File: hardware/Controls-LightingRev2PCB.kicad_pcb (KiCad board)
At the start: 2 copper layers, 54.5 x 53.5 mm, 52 parts, among them IC1 LM74502HDDFR, IC3 ACS724LLCTR-05AU-T, IC4 ACS724LLCTR-05AU-T, IC5 TLV70433DBVT, IC6 ACS724LLCTR-05AU-T, J1 53307-2471, J3 Conn_02x05_Top_Bottom, J4 Conn_01x02, J5 Conn_01x02, J6 Conn_01x03, Q1 NVMFWS1D7N04XMT1G, Q3 IRLML0030, Q4 NVMFWS1D7N04XMT1G, Q5 IRLML0030, U5 SN74LV1T34DBV

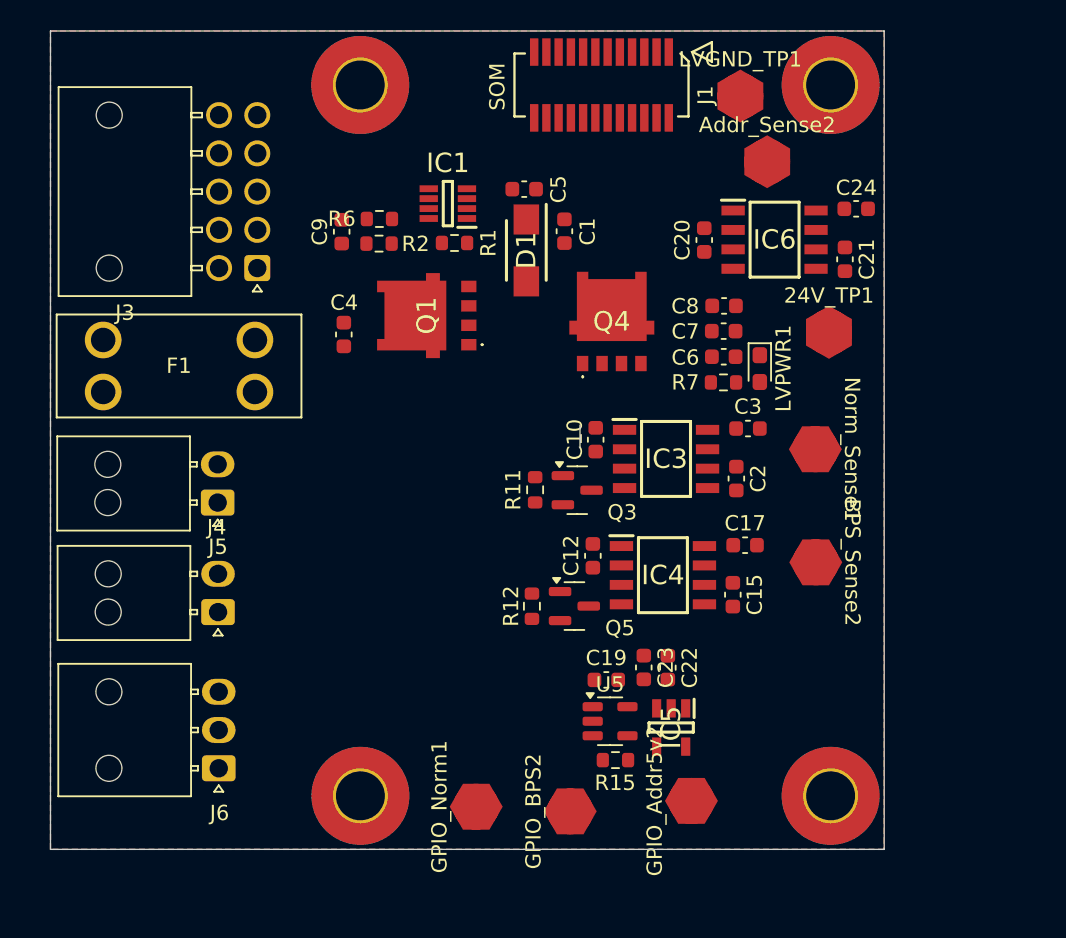
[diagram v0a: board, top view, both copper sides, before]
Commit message: Some routing
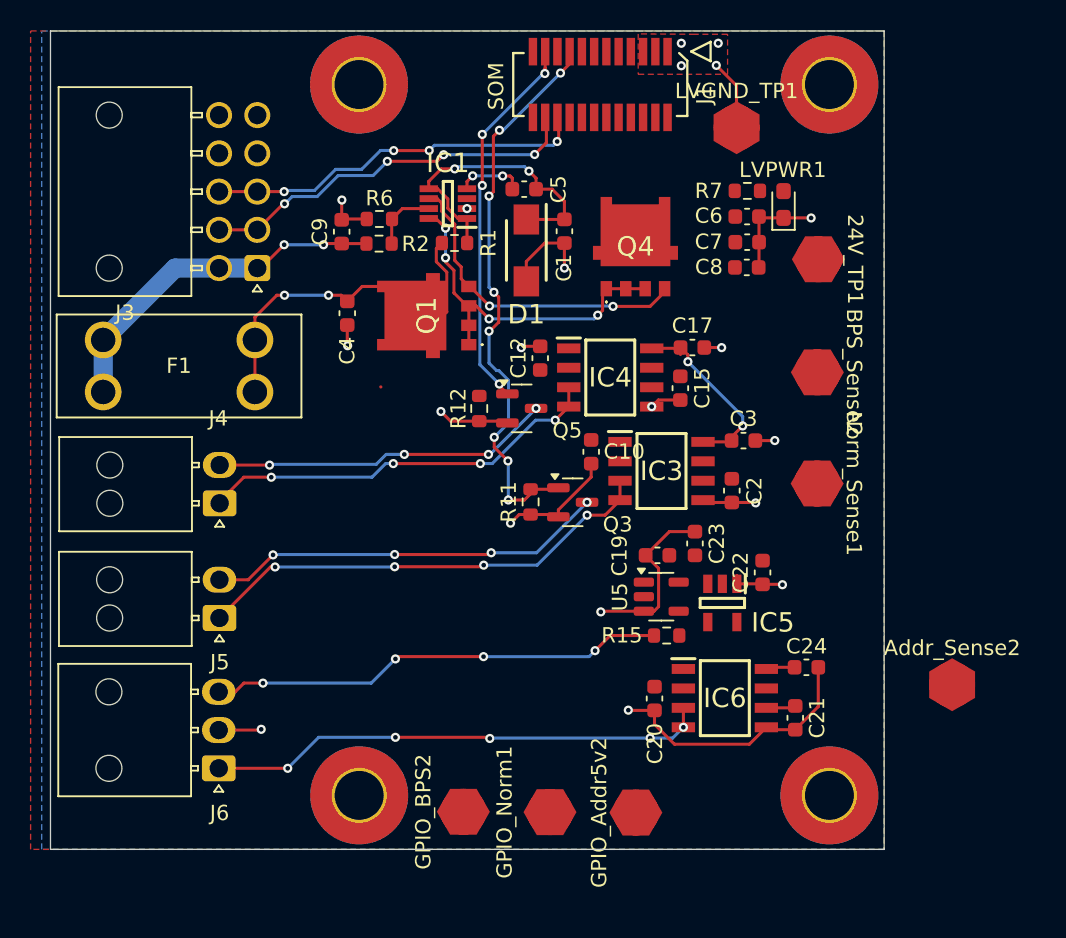
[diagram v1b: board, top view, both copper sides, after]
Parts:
- moved Addr_Sense2 36.3 mm to (232.9, 127.7)
- moved C20 30.1 mm to (213.5, 128.6)
- moved C24 30.1 mm to (223.4, 126.6)
- moved C21 30.1 mm to (222.7, 129.9)
- moved IC6 30.1 mm to (218.1, 128.6)
- moved C15 13.9 mm to (215.2, 108.3)
- moved R12 13.4 mm to (202.0, 109.7)
- moved C12 13.4 mm to (206.0, 106.4)
- moved C17 13.4 mm to (216.0, 105.7)
- moved IC4 13.4 mm to (210.6, 107.7)
- moved Q5 13.4 mm to (204.8, 109.7)
- moved R7 12.6 mm to (219.6, 95.5), turned to 0 degrees
- moved BPS_Sense2 12.4 mm to (224.1, 107.3)
- moved LVPWR1 10.8 mm to (221.9, 96.3), turned to 90 degrees
- moved C6 9.29 mm to (219.5, 97.1), turned to 0 degrees
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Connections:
- 24V_TP1 pad 1: Addressable_PWR -> +24V
- C1 pad 1: Addressable_GND -> GND
- C10 pad 1: Addressable_GND -> GND
- C10 pad 2: Addressable_PWR -> +24V
- C12 pad 1: Addressable_GND -> GND
- C12 pad 2: Addressable_PWR -> +24V
- C15 pad 2: Addressable_GND -> GND
- C17 pad 2: Addressable_GND -> GND
- C19 pad 1: Addressable_GND -> GND
- C2 pad 2: Addressable_GND -> GND
- C20 pad 1: Addressable_GND -> GND
- C20 pad 2: Addressable_PWR -> +24V
- C21 pad 2: Addressable_GND -> GND
- C22 pad 1: Addressable_GND -> GND
- C22 pad 2: Addressable_PWR -> +24V
- C23 pad 1: Addressable_GND -> GND
- C24 pad 2: Addressable_GND -> GND
- C3 pad 2: Addressable_GND -> GND
- C4 pad 2: Addressable_GND -> GND
- C6 pad 1: Addressable_PWR -> +24V
- C6 pad 2: Addressable_GND -> GND
- C7 pad 1: Addressable_PWR -> +24V
- C7 pad 2: Addressable_GND -> GND
- C8 pad 1: Addressable_PWR -> +24V
- C8 pad 2: Addressable_GND -> GND
- C9 pad 2: Addressable_GND -> GND
- D1 pad 2: Addressable_GND -> GND
- IC1 pad 2: Addressable_GND -> GND
- IC3 pad 1: Addressable_PWR -> +24V
- IC3 pad 2: Addressable_PWR -> +24V
- IC3 pad 3: Normal_GND -> Net-(IC3-IP-_1)
- IC3 pad 4: Normal_GND -> Net-(IC3-IP-_1)
- IC3 pad 5: Addressable_GND -> GND
- IC4 pad 1: Addressable_PWR -> +24V
- IC4 pad 2: Addressable_PWR -> +24V
- IC4 pad 3: Strobe_GND -> Net-(IC4-IP-_1)
- IC4 pad 4: Strobe_GND -> Net-(IC4-IP-_1)
- IC4 pad 5: Addressable_GND -> GND
- IC5 pad 1: Addressable_GND -> GND
- IC5 pad 2: Addressable_PWR -> +24V
- IC6 pad 1: Addressable_PWR -> +24V
- IC6 pad 2: Addressable_PWR -> +24V
- IC6 pad 3: Addressable_GND -> Net-(IC6-IP-_1)
- IC6 pad 4: Addressable_GND -> Net-(IC6-IP-_1)
- IC6 pad 5: Addressable_GND -> GND
- J1 pad 1: Addressable_GND -> GND
- J1 pad 24: Addressable_PWR -> +24V
- J1 pad 3: Addressable_GND -> GND
- J1 pad 5: Addressable_GND -> GND
- J3 pad 10: Addressable_GND -> GND
- J3 pad 4: Addressable_GND -> GND
- J3 pad 5: Addressable_GND -> GND
- J3 pad 9: Addressable_GND -> GND
- J4 pad 1: Addressable_PWR -> Net-(IC4-IP-_1)
- J4 pad 2: Strobe_GND -> Net-(J4-Pin_2)
- J5 pad 1: Addressable_PWR -> Net-(IC3-IP-_1)
- J5 pad 2: Normal_GND -> Net-(J5-Pin_2)
- J6 pad 1: Addressable_PWR -> Net-(IC6-IP-_1)
- J6 pad 2: Addressable_GND -> GND
- LVGND_TP1 pad 1: Addressable_GND -> GND
- LVPWR1 pad 1: Addressable_GND -> GND
- Q3 pad 2: Addressable_GND -> GND
- Q3 pad 3: Normal_GND -> Net-(J5-Pin_2)
- Q4 pad 5: Addressable_PWR -> +24V
- Q4 pad 6: Addressable_PWR -> +24V
- Q4 pad 7: Addressable_PWR -> +24V
- Q4 pad 8: Addressable_PWR -> +24V
- Q4 pad 9: Addressable_PWR -> +24V
- Q5 pad 2: Addressable_GND -> GND
- Q5 pad 3: Strobe_GND -> Net-(J4-Pin_2)
- R11 pad 1: Addressable_GND -> GND
- R12 pad 1: Addressable_GND -> GND
- R6 pad 2: Addressable_GND -> GND
- R7 pad 1: Addressable_PWR -> +24V
- U5 pad 3: Addressable_GND -> GND
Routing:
- net GND: track 0.00 -> 78.8 mm, vias 0 -> 20
- net GPIO_Normal: track 0.00 -> 37.4 mm, vias 0 -> 8
- net Net-(IC6-IP-_1): track 0.00 -> 32.9 mm, vias 0 -> 5
- net Net-(IC3-IP-_1): track 0.00 -> 30.6 mm, vias 0 -> 4
- net Addressable_Logic: track 0.00 -> 30.0 mm, vias 0 -> 4
- net Net-(IC4-IP-_1): track 0.00 -> 27.2 mm, vias 0 -> 4
- net Net-(J5-Pin_2): track 0.00 -> 26.1 mm, vias 0 -> 4
- net CAN_H: track 0.00 -> 25.8 mm, vias 0 -> 4
- net CAN_L: track 0.00 -> 25.1 mm, vias 0 -> 4
- net GPIO_BPS_Strobe: track 0.00 -> 25.0 mm, vias 0 -> 4
- net 24V_EXT: track 0.00 -> 23.3 mm, vias 0 -> 2
- net Net-(IC1-SRC): track 0.00 -> 23.1 mm, vias 0 -> 4
- net Net-(J4-Pin_2): track 0.00 -> 22.2 mm, vias 0 -> 4
- net Net-(IC1-GATE): track 0.00 -> 21.2 mm, vias 0 -> 2
- net /Reverse Polarity Protection/RPP_EN: track 0.00 -> 20.1 mm, vias 0 -> 2
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- added copper zone on F.Cu, net +24V
- added copper zone on B.Cu, net GND
- added copper zone on F.Cu, net GND
- removed copper zone on B.Cu, net Addressable_GND
- removed copper zone on F.Cu, net Addressable_PWR
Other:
- outline, holes or cut-outs redrawn
